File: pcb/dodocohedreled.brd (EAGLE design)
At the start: 50 x 47.5 mm, 11 parts

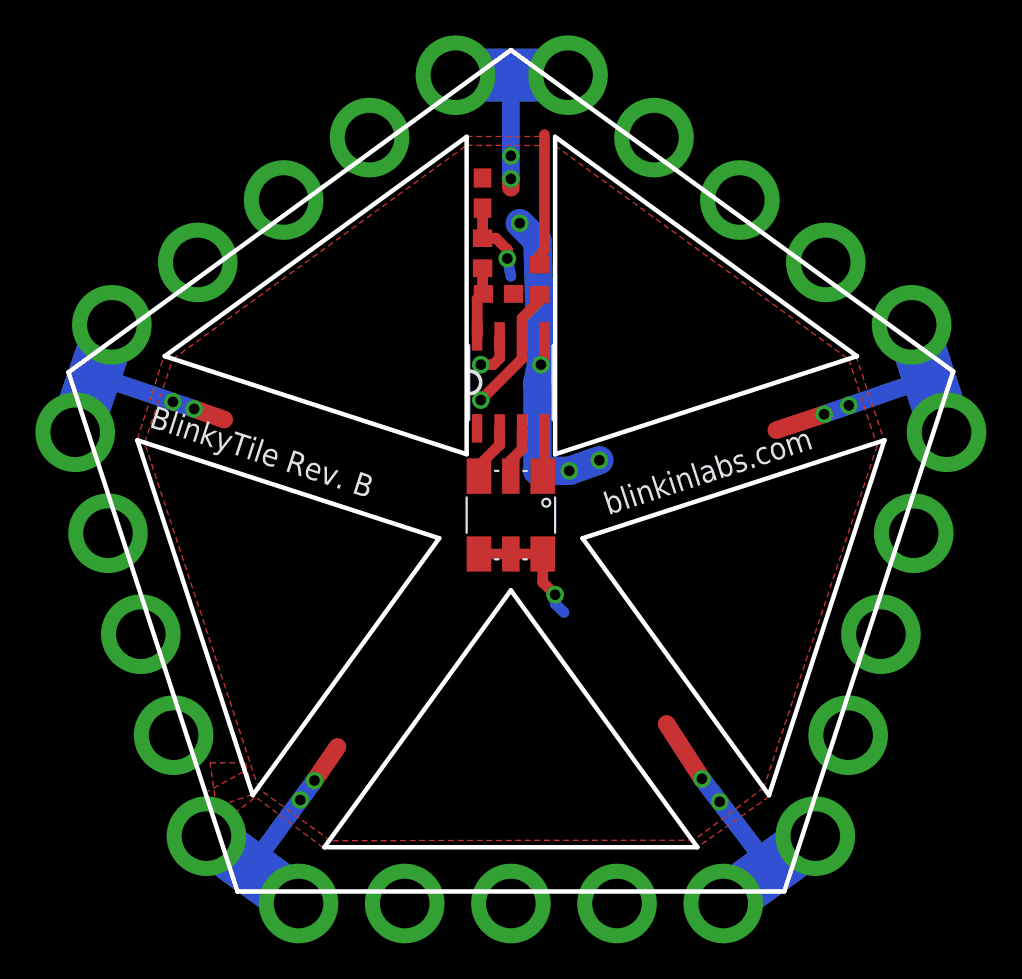
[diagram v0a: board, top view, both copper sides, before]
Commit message: Update for RevC
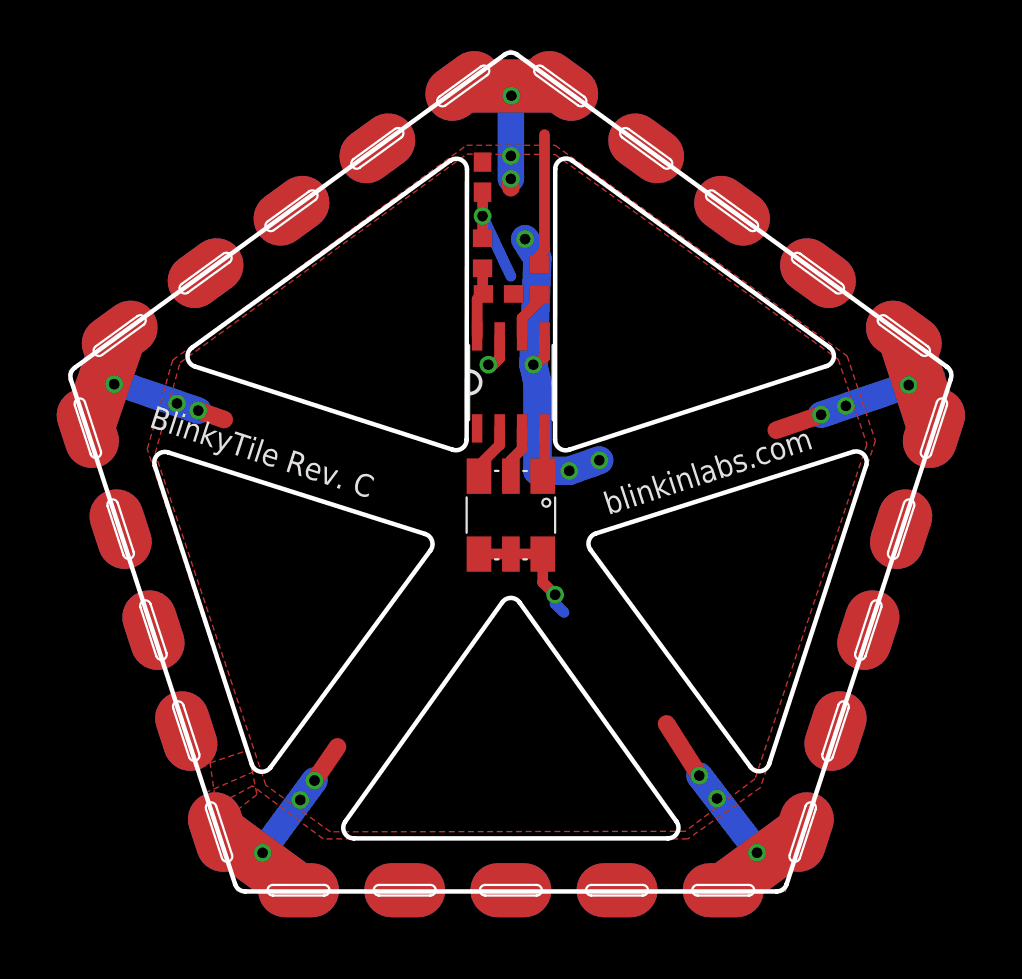
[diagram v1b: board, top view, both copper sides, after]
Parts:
- U$2, U$3, U$4, U$5, U$6: value D_EDGE -> D_EDGESLOT; device dodocohedreled:D_EDGE -> dodocohedreled:D_EDGE_SLOT
- moved C2 0.90 mm to (-1.60, 19.1)
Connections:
- net 5V: now also U$2.P$7, U$2.P$9, U$3.P$7, U$3.P$9, U$4.P$7, U$4.P$9, U$5.P$7, U$5.P$9, U$6.P$7, U$6.P$9
- net DATA: now also U$2.P$8, U$3.P$8, U$4.P$8, U$5.P$8, U$6.P$8
- net GND: now also U$2.P$10, U$2.P$6, U$3.P$10, U$3.P$6, U$4.P$10, U$4.P$6, U$5.P$10, U$5.P$6, U$6.P$10, U$6.P$6
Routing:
- net GND: track 109.7 -> 130.3 mm, vias 14 -> 19
- net N$10: track 7.30 -> 2.73 mm, vias 1 -> 0
- net 5V: track 12.3 -> 13.8 mm
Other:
- board size 50 x 47.5 mm -> 49.8 x 47.4 mm
- board text added: "BlinkyTile Rev. C"
- board text removed: "BlinkyTile Rev. B"
